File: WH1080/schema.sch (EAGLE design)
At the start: 19 parts

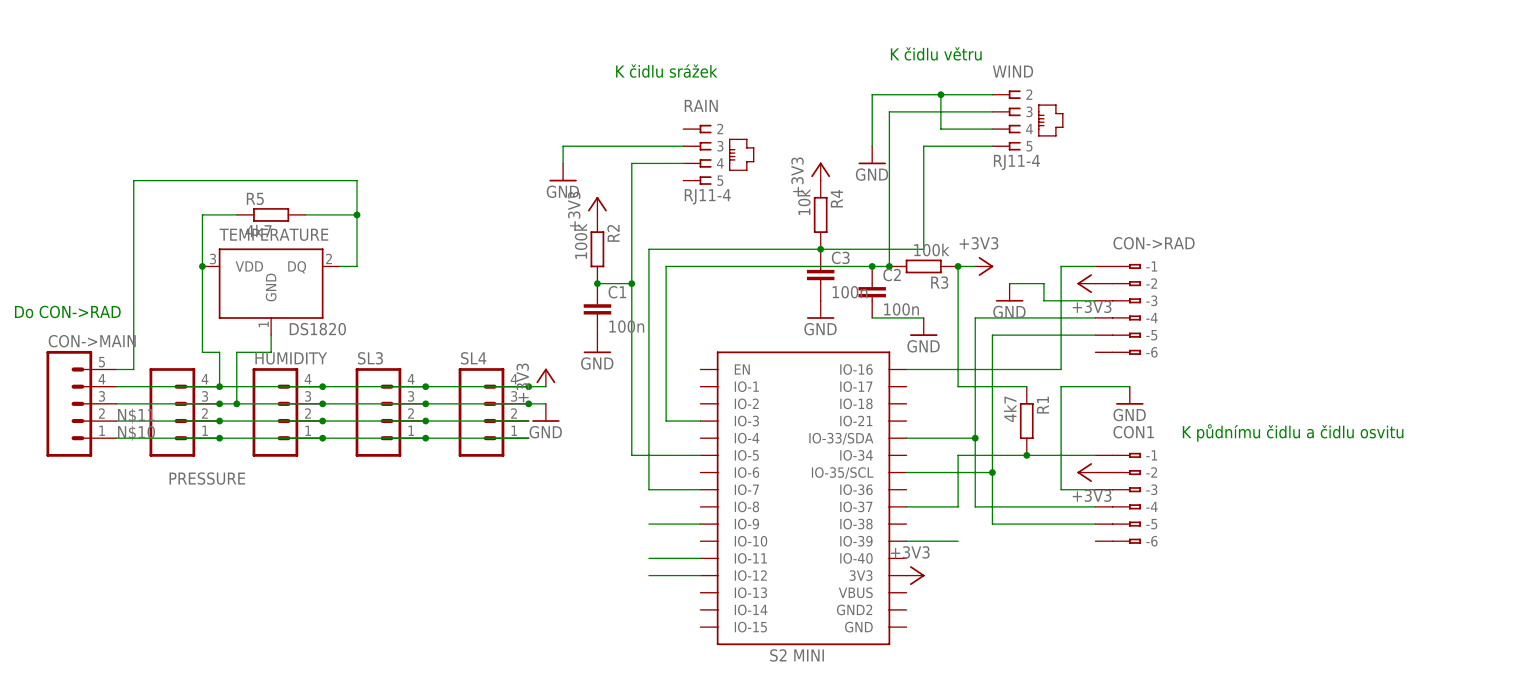
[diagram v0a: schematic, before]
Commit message: vyroba DPS
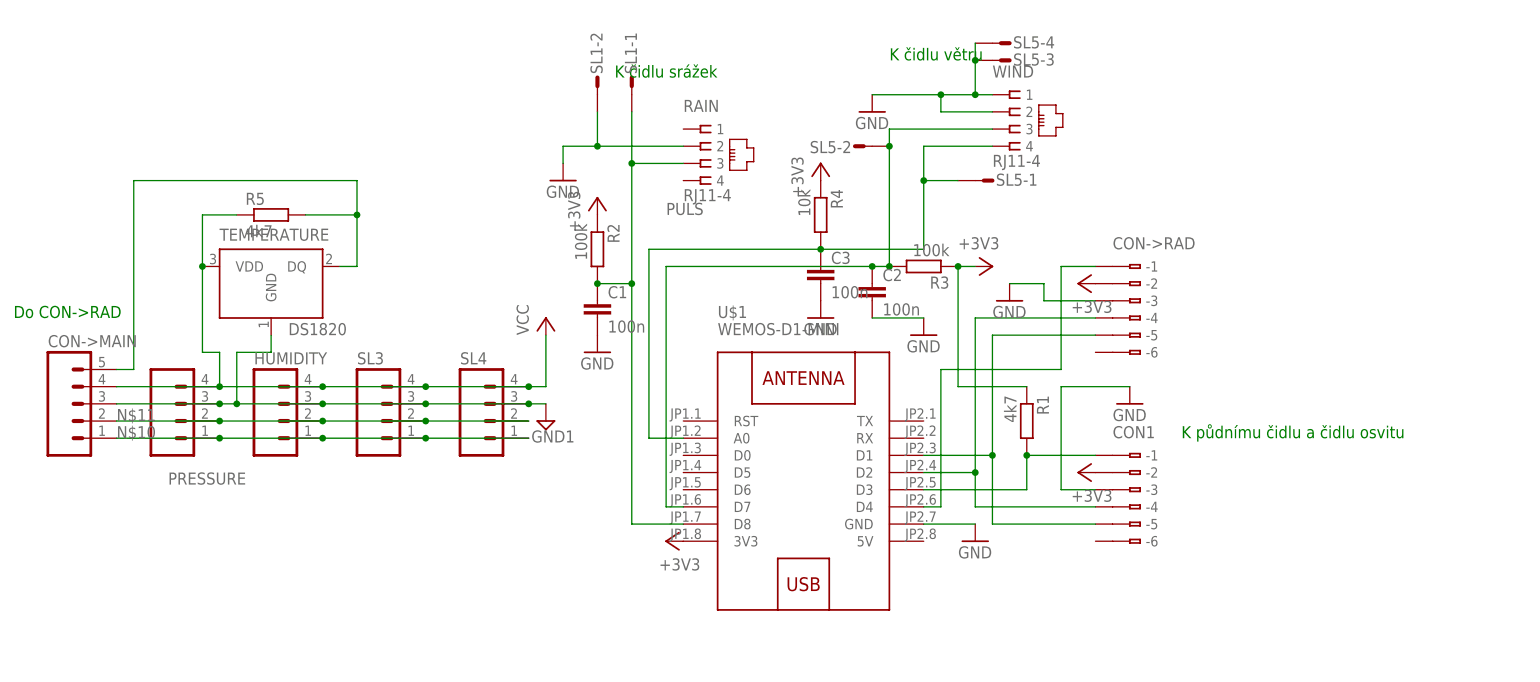
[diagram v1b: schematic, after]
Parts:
- added SL1: (no value), con-amp-quick:M02S
- added SL5: (no value), con-amp-quick:M04S
- U$1: value WEMOS_S2_MINI -> WEMOS-D1-MINI; device Wemos_Boards:WEMOS_S2_MINI -> Wemos_Boards:WEMOS-D1-MINI
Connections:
- removed net N$1: C1.1, R2.2, RAIN.4, U$1.IO-5
- removed net N$12: U$1.IO-39
- removed net N$15: U$1.IO-12
- removed net N$16: U$1.IO-11
- removed net N$17: U$1.IO-9
- removed net N$2: C3.1, R4.2, U$1.IO-7, WIND.5
- removed net N$4: C2.1, R3.2, U$1.IO-3, WIND.3
- new net GND1: CON->MAIN.3, HUMIDITY.3, PRESSURE.3, SL3.3, SL4.3, TEMPERATURE.GND
- new net PULS: C1.1, R2.2, RAIN.3, SL1-1.S, U$1.D8
- new net RYCHLOST: C2.1, R3.2, SL5-2.S, U$1.D7, WIND.3
- new net SMER: C3.1, R4.2, SL5-1.S, U$1.A0, WIND.4
- new net VCC: CON->MAIN.4, HUMIDITY.4, PRESSURE.4, R5.1, SL3.4, SL4.4, TEMPERATURE.VDD
- net +3V3: no longer CON->MAIN.4, HUMIDITY.4, PRESSURE.4, R5.1, SL3.4, SL4.4, TEMPERATURE.VDD
- net GND: now also RAIN.2, SL1-2.S, SL5-3.S, SL5-4.S, U$1.GND, WIND.1; no longer CON->MAIN.3, HUMIDITY.3, PRESSURE.3, RAIN.3, SL3.3, SL4.3, TEMPERATURE.GND, WIND.4
- net N$13: now also U$1.D3; no longer U$1.IO-37
- net N$14: now also U$1.D4; no longer U$1.IO-16
- net SCL: now also U$1.D1; no longer U$1.IO-35/SCL
- net SDA: now also U$1.D2; no longer U$1.IO-33/SDA
